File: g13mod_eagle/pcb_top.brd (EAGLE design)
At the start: 85.2 x 17.3 mm, 20 parts

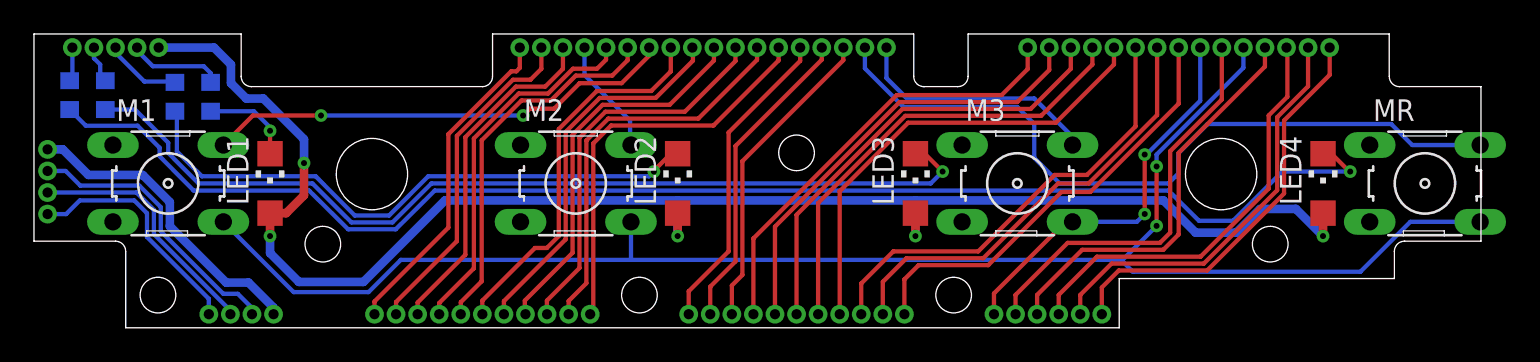
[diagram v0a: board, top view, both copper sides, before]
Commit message: Fix bug
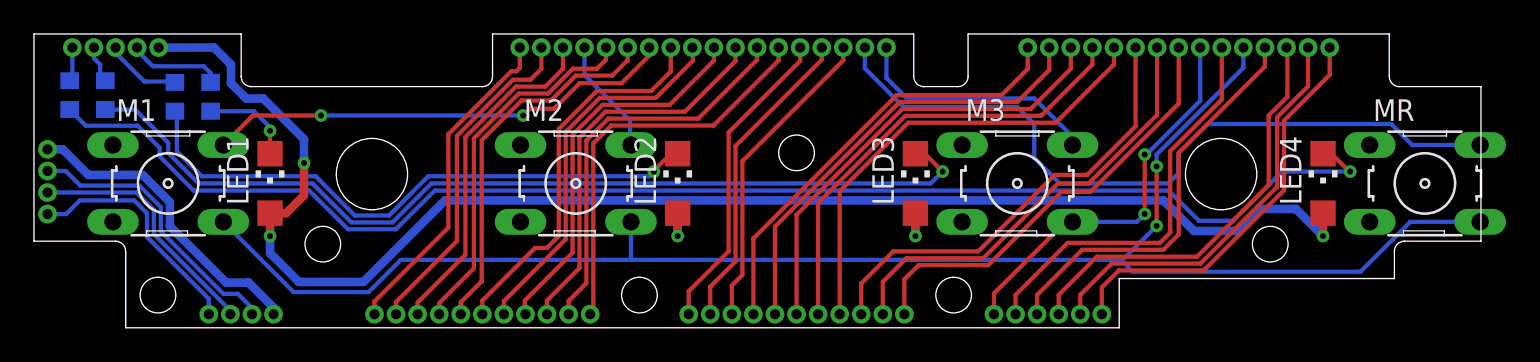
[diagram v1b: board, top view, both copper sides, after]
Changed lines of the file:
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@@
 <contactref element="LED3" pad="A"/>
 <contactref element="LED2" pad="A"/>
-<wire x1="31" y1="-1.75" x2="31" y2="-1.7" width="0.508" layer="1"/>
 <wire x1="31" y1="-1.75" x2="31" y2="-3.1" width="0.508" layer="1"/>
 <via x="31" y="-3.1" extent="1-16" drill="0.35"/>
@@
 <via x="-7" y="-3.1" extent="1-16" drill="0.35"/>
 <wire x1="-7" y1="-3.1" x2="-7" y2="-1" width="0.508" layer="16"/>
-<wire x1="21.6" y1="-1" x2="23.5" y2="-2.9" width="0.508" layer="16"/>
+<wire x1="21.6" y1="-1" x2="23.4" y2="-2.8" width="0.508" layer="16"/>
 <wire x1="-7" y1="-1" x2="7" y2="-1" width="0.508" layer="16"/>
 <wire x1="7" y1="-1" x2="21.6" y2="-1" width="0.508" layer="16"/>
@@
 <wire x1="-32.4" y1="5" x2="-31.4" y2="5" width="0.508" layer="16"/>
 <wire x1="-37.56" y1="8" x2="-34.3" y2="8" width="0.508" layer="16"/>
-<wire x1="23.5" y1="-2.9" x2="25.9" y2="-2.9" width="0.508" layer="16"/>
-<wire x1="25.9" y1="-2.9" x2="27.3" y2="-1.5" width="0.508" layer="16"/>
-<wire x1="27.3" y1="-1.5" x2="29.4" y2="-1.5" width="0.508" layer="16"/>
+<wire x1="23.4" y1="-2.8" x2="25.9" y2="-2.8" width="0.508" layer="16"/>
+<wire x1="25.9" y1="-2.8" x2="27.2" y2="-1.5" width="0.508" layer="16"/>
+<wire x1="27.2" y1="-1.5" x2="29.4" y2="-1.5" width="0.508" layer="16"/>
 <wire x1="29.4" y1="-1.5" x2="31" y2="-3.1" width="0.508" layer="16"/>
 </signal>
@@
 <contactref element="R2" pad="1"/>
 <contactref element="JP3" pad="3"/>
-<wire x1="-40.1" y1="8" x2="-40.1" y2="7.55" width="0.254" layer="16"/>
 <wire x1="-40.1" y1="8" x2="-40.1" y2="7.7" width="0.254" layer="16"/>
 <wire x1="-38.4" y1="6" x2="-40.1" y2="7.7" width="0.254" layer="16"/>
@@
 <contactref element="R3" pad="1"/>
 <contactref element="JP3" pad="2"/>
-<wire x1="-40.77" y1="6.12" x2="-40.7" y2="6.05" width="0.254" layer="16"/>
 <wire x1="-41.37" y1="8" x2="-41.37" y2="7.37" width="0.254" layer="16"/>
 <wire x1="-41" y1="7" x2="-41.37" y2="7.37" width="0.254" layer="16"/>
@@
 <wire x1="17.1" y1="0.5" x2="15.2" y2="0.5" width="0.254" layer="1"/>
 <contactref element="JP2" pad="3"/>
-<wire x1="3.81" y1="-7.7" x2="3.81" y2="-7.49" width="0.254" layer="1"/>
 <wire x1="3.81" y1="-7.7" x2="3.81" y2="-5.89" width="0.254" layer="1"/>
 <wire x1="3.81" y1="-5.89" x2="5.7" y2="-4" width="0.254" layer="1"/>
@@
 <wire x1="28.9" y1="5.1" x2="28.9" y2="7.95" width="0.254" layer="1"/>
 <wire x1="28.9" y1="7.95" x2="28.85" y2="8" width="0.254" layer="1"/>
-<wire x1="27.8" y1="-0.3" x2="27.8" y2="4" width="0.254" layer="1"/>
-<wire x1="23.7872" y1="-4.3128" x2="27.8" y2="-0.3" width="0.254" layer="1"/>
-<wire x1="23.7872" y1="-4.3128" x2="17.6872" y2="-4.3128" width="0.254" layer="1"/>
+<wire x1="27.8" y1="-0.1" x2="27.8" y2="4" width="0.254" layer="1"/>
+<wire x1="23.5872" y1="-4.3128" x2="27.8" y2="-0.1" width="0.254" layer="1"/>
+<wire x1="23.5872" y1="-4.3128" x2="17.6872" y2="-4.3128" width="0.254" layer="1"/>
 <contactref element="JP1" pad="3"/>
 <wire x1="17.6872" y1="-4.3128" x2="15.435" y2="-6.565" width="0.254" layer="1"/>
@@
 <wire x1="30.12" y1="8" x2="30.12" y2="5.72" width="0.254" layer="1"/>
 <wire x1="30.12" y1="5.72" x2="28.3" y2="3.9" width="0.254" layer="1"/>
-<wire x1="28.3" y1="3.9" x2="28.3" y2="-0.4" width="0.254" layer="1"/>
-<wire x1="23.9808" y1="-4.7192" x2="28.3" y2="-0.4" width="0.254" layer="1"/>
-<wire x1="23.9808" y1="-4.7192" x2="18.5508" y2="-4.7192" width="0.254" layer="1"/>
+<wire x1="28.3" y1="3.9" x2="28.3" y2="-0.2" width="0.254" layer="1"/>
+<wire x1="23.7808" y1="-4.7192" x2="28.3" y2="-0.2" width="0.254" layer="1"/>
+<wire x1="23.7808" y1="-4.7192" x2="18.5508" y2="-4.7192" width="0.254" layer="1"/>
 <contactref element="JP1" pad="2"/>
 <wire x1="18.5508" y1="-4.7192" x2="16.705" y2="-6.565" width="0.254" layer="1"/>
@@
 <wire x1="31.39" y1="6.39" x2="31.39" y2="8" width="0.254" layer="1"/>
 <wire x1="28.7064" y1="3.7064" x2="31.39" y2="6.39" width="0.254" layer="1"/>
-<wire x1="28.7064" y1="-0.5936" x2="28.7064" y2="3.7064" width="0.254" layer="1"/>
-<wire x1="24.1744" y1="-5.1256" x2="28.7064" y2="-0.5936" width="0.254" layer="1"/>
-<wire x1="24.1744" y1="-5.1256" x2="18.9744" y2="-5.1256" width="0.254" layer="1"/>
+<wire x1="28.7064" y1="-0.3936" x2="28.7064" y2="3.7064" width="0.254" layer="1"/>
+<wire x1="23.9744" y1="-5.1256" x2="28.7064" y2="-0.3936" width="0.254" layer="1"/>
+<wire x1="23.9744" y1="-5.1256" x2="18.9744" y2="-5.1256" width="0.254" layer="1"/>
 <contactref element="JP1" pad="1"/>
 <wire x1="18.9744" y1="-5.1256" x2="17.975" y2="-6.125" width="0.254" layer="1"/>
